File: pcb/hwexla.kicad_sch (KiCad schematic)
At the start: 34 parts, among them J1 DB25_Male, J2 Conn_01x03, J3 AVR-ISP-6, J4 Conn_01x06, SW1 SW_Push, U1 ATmega8A-AU, U2 RR112-1

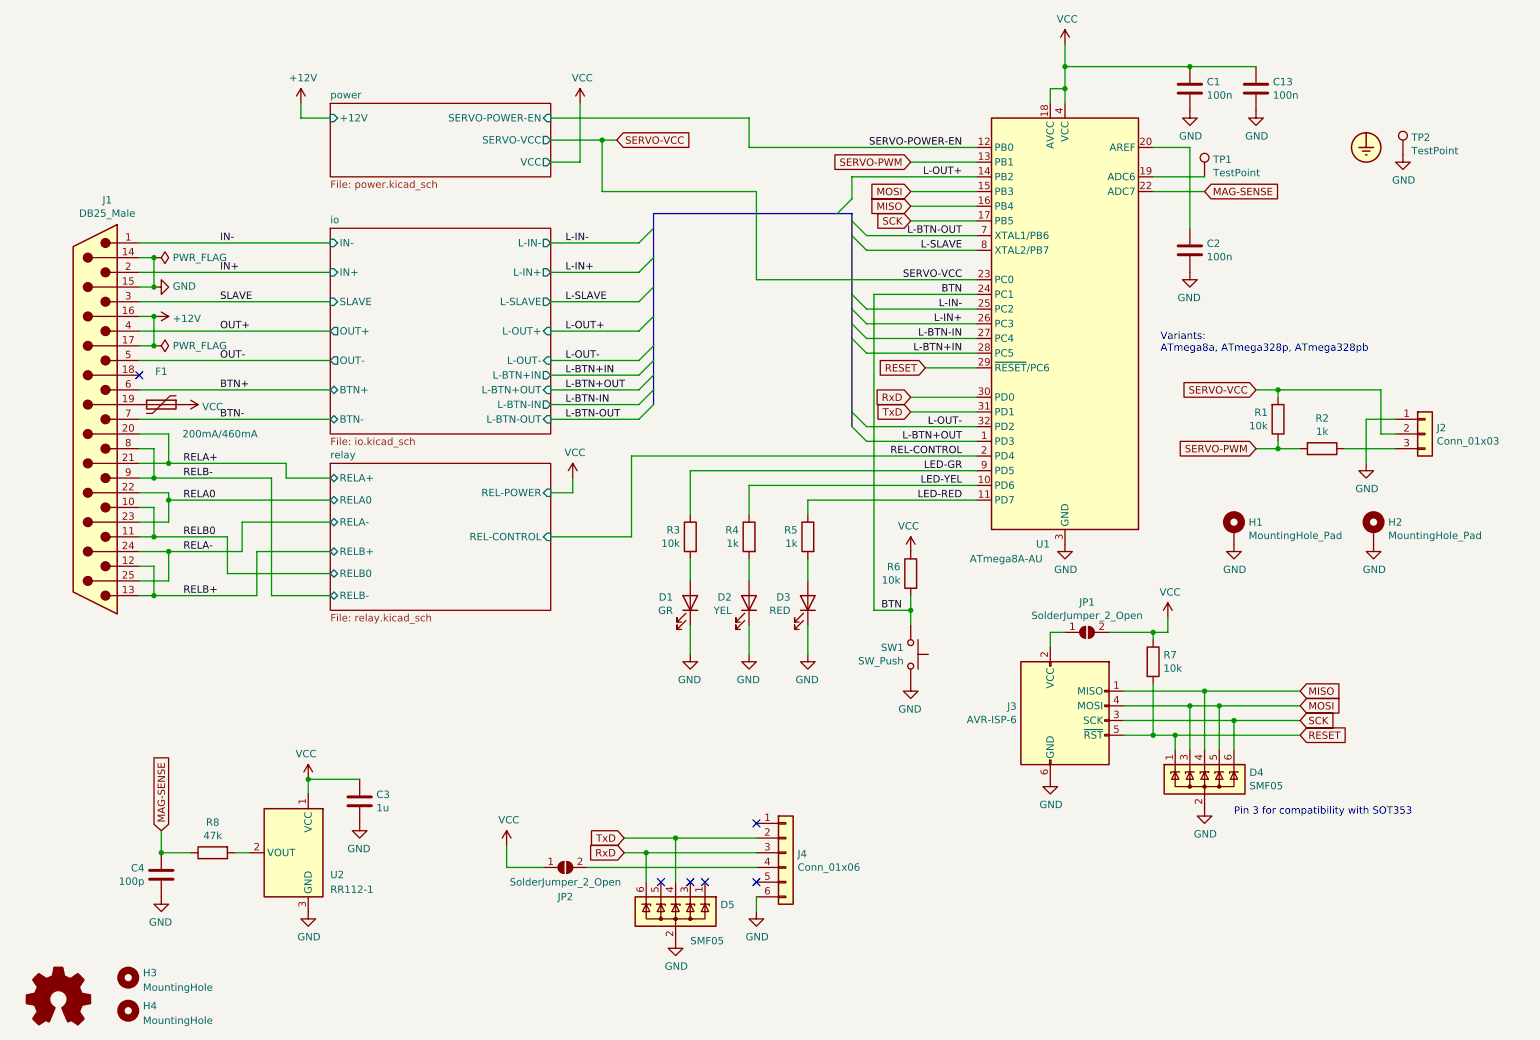
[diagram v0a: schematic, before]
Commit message: Add protection on internal inputs, divide stepdown voltage measuring by 2.
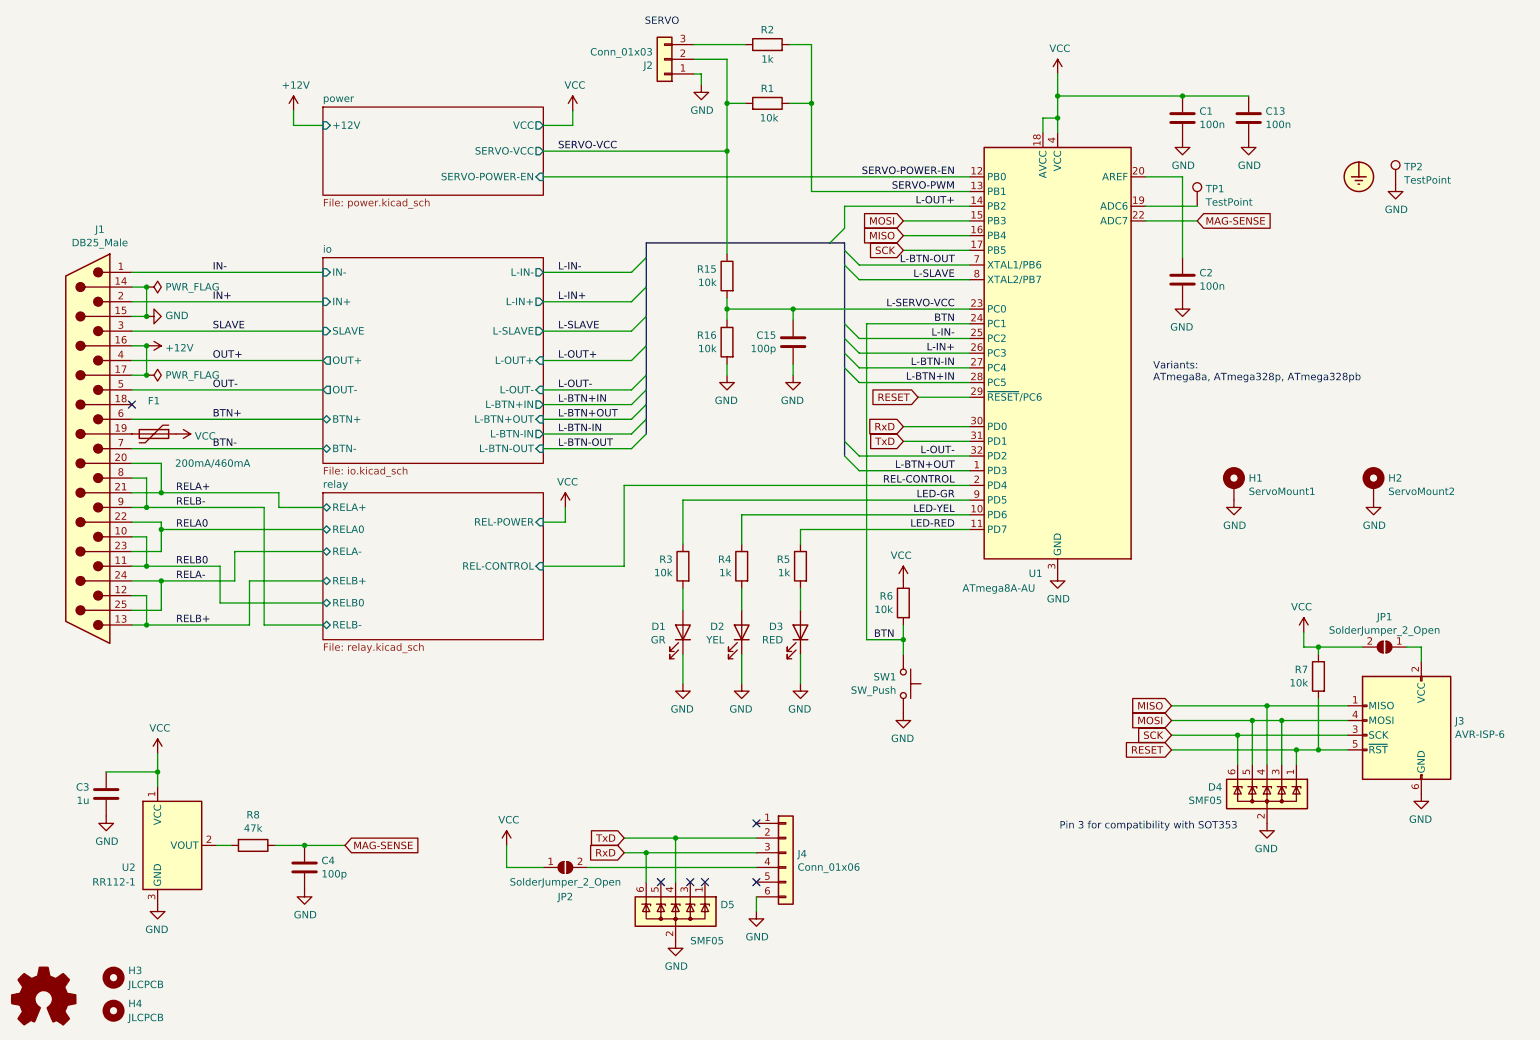
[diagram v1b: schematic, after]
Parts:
- added C15: 100p, Capacitor_SMD:C_0805_2012Metric_Pad1.18x1.45mm_HandSolder, symbol Device:C
- added R15, R16: 10k, Resistor_SMD:R_0805_2012Metric_Pad1.20x1.40mm_HandSolder, symbol Device:R
- H1: value MountingHole_Pad -> ServoMount1
- H2: value MountingHole_Pad -> ServoMount2
- H3, H4: value MountingHole -> JLCPCB
- J1: symbol Connector:DB25_Male -> Connector:DB25_Plug
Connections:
- net GND: now also C15.2, R16.2
- net SERVO-VCC: now also R15.1; no longer U1.23 (PC0)
- new net L-SERVO-VCC: C15.1, R15.2, R16.1, U1.23 (PC0)
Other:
- note added: "SERVO"
- moved on the sheet: C1, C13, C2, C3, C4, D1, D2, D3, D4, F1, H1, H2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
